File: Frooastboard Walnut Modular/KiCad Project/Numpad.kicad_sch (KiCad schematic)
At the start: 63 parts, among them J19 Conn_01x15_Pin, J20 Conn_01x06_Male, J21 Conn_01x13_Male, M1 Frooastboard_MM2040

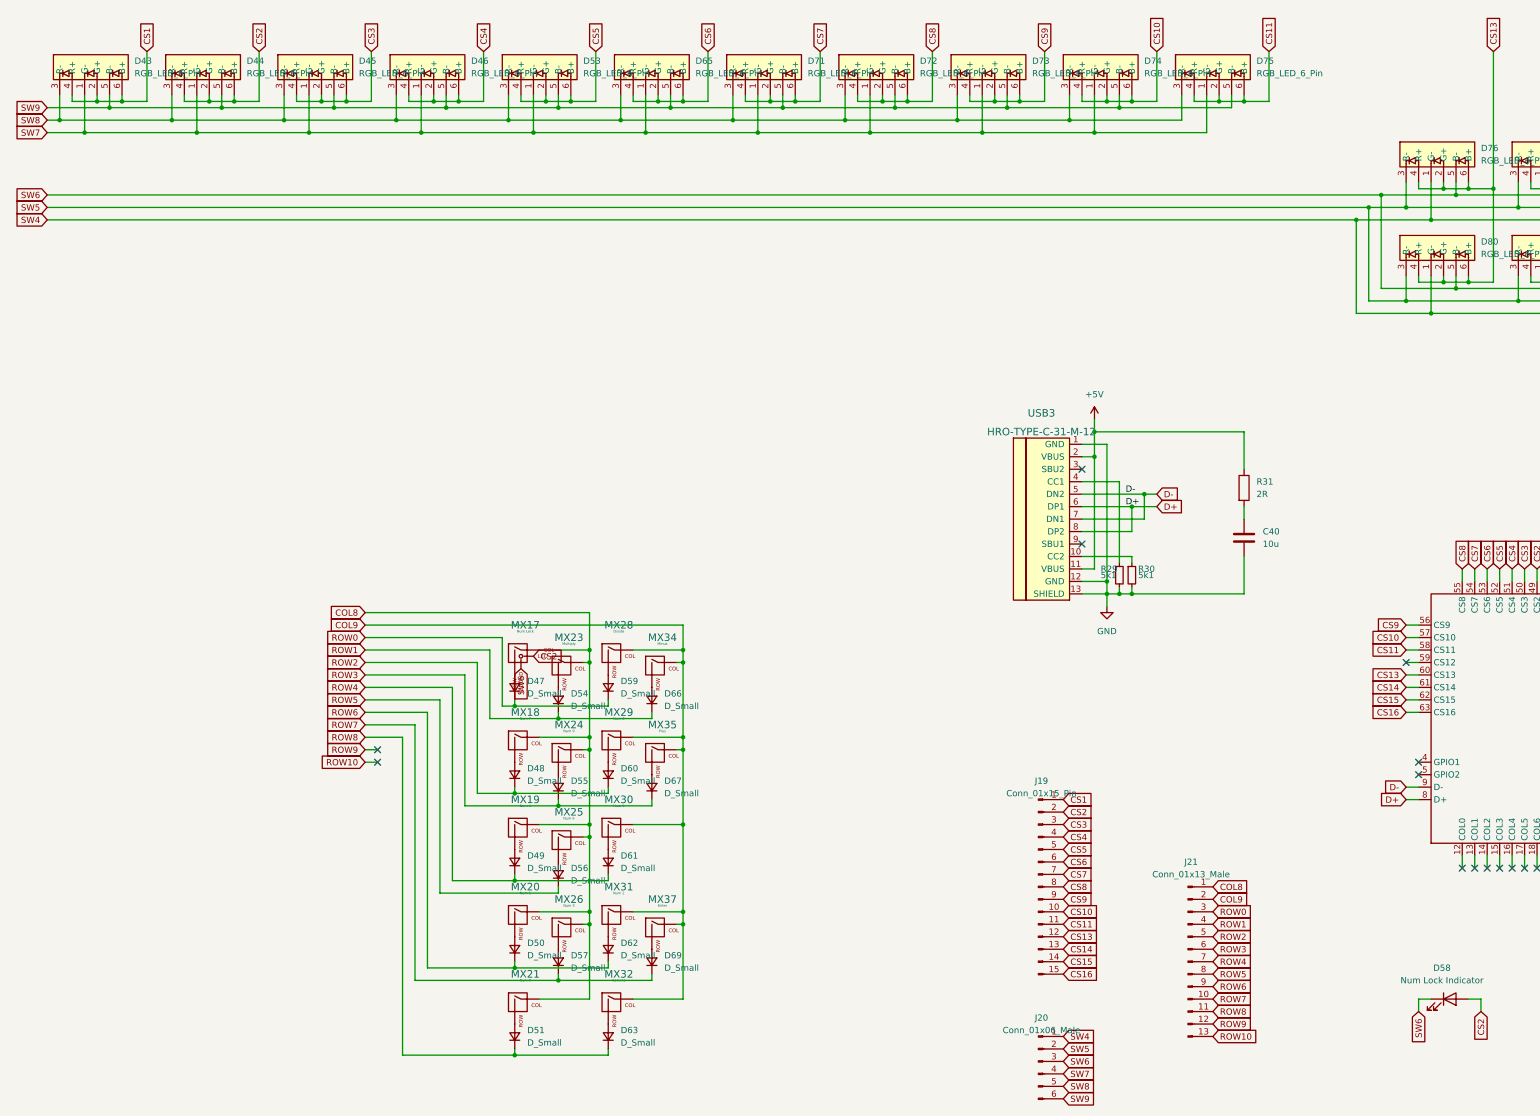
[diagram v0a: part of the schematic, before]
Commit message: updates or something like that
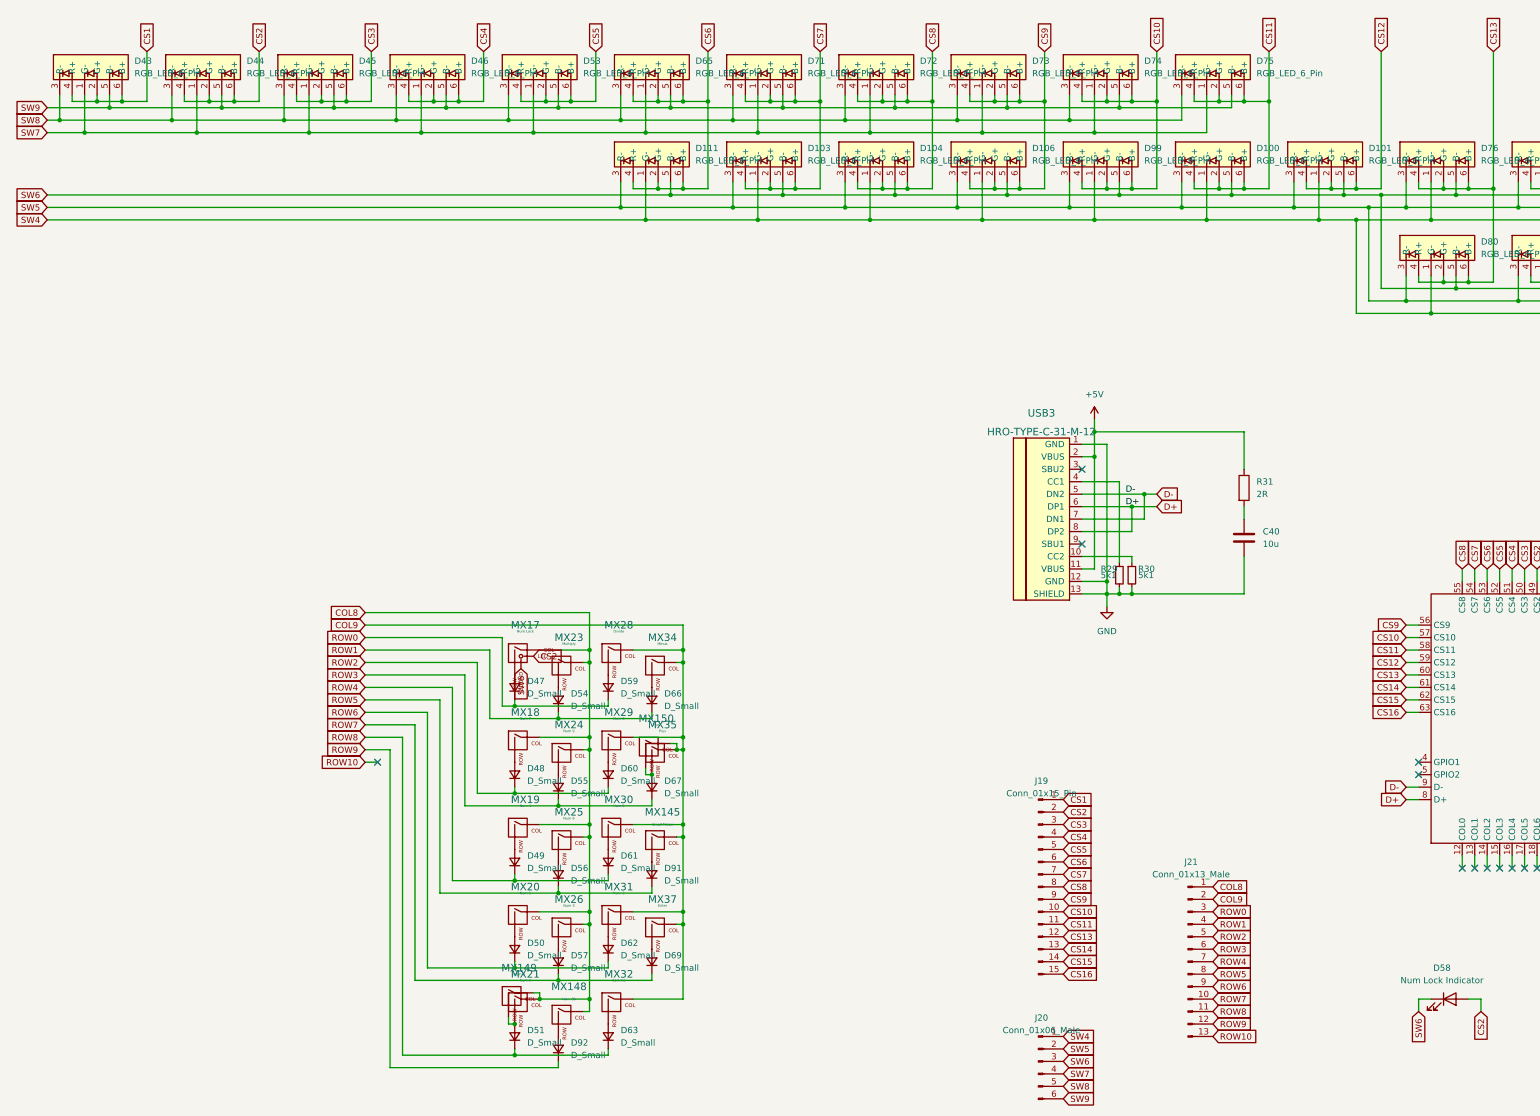
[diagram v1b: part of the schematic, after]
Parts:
- added D100, D101, D103, D104, D106, D111, D99: RGB_LED_6_Pin, Frooastboard Footprints:Everlight 99-235, symbol Frooastboard Symbols:RGB_LED_6_Pin
- added D91, D92: D_Small, Diode_SMD:D_0805_2012Metric, symbol Device:D_Small
- added MX145: Small Minus, MX_Only:MXOnly-1U-NoLED, symbol MX_Alps_Hybrid:MX-NoLED
- added MX148: Num 00, MX_Only:MXOnly-1U-NoLED, symbol MX_Alps_Hybrid:MX-NoLED
- added MX149: Num 0, MX_Only:MXOnly-1U-NoLED, symbol MX_Alps_Hybrid:MX-NoLED
- added MX150: Plus, MX_Only:MXOnly-1U-NoLED, symbol MX_Alps_Hybrid:MX-NoLED
- MX35, MX37: footprint MX_Only:MXOnly-2U-VerticalStabilizers-NoLED -> MX_Only:MXOnly-2U-ReversedVerticalStabilizers-NoLED
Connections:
- net COL8: now also MX148.1 (COL), MX149.1 (COL)
- net COL9: now also MX145.1 (COL), MX150.1 (COL)
- net CS10: now also D99.2 (G+), D99.4 (R+), D99.6 (B+)
- net CS11: now also D100.2 (G+), D100.4 (R+), D100.6 (B+)
- net CS6: now also D111.2 (G+), D111.4 (R+), D111.6 (B+)
- net CS7: now also D103.2 (G+), D103.4 (R+), D103.6 (B+)
- net CS8: now also D104.2 (G+), D104.4 (R+), D104.6 (B+)
- net CS9: now also D106.2 (G+), D106.4 (R+), D106.6 (B+)
- net ROW5: now also D91.1 (K)
- net ROW9: now also D92.1 (K)
- net SW4: now also D100.1 (G-), D101.1 (G-), D103.1 (G-), D104.1 (G-), D106.1 (G-), D111.1 (G-), D99.1 (G-)
- net SW5: now also D100.3 (R-), D101.3 (R-), D103.3 (R-), D104.3 (R-), D106.3 (R-), D111.3 (R-), D99.3 (R-)
- net SW6: now also D100.5 (B-), D101.5 (B-), D103.5 (B-), D104.5 (B-), D106.5 (B-), D111.5 (B-), D99.5 (B-)
- net at D51.2 (A), MX21.2 (ROW): now also MX149.2 (ROW)
- net CS12: now reaches M1.59 (CS12)
- net CS12: now also D101.2 (G+), D101.4 (R+), D101.6 (B+)
- net at D67.2 (A), MX35.2 (ROW): now also MX150.2 (ROW)
- new net: D92.2 (A), MX148.2 (ROW)
- new net: D91.2 (A), MX145.2 (ROW)
- no-connect marks 22 -> 20
